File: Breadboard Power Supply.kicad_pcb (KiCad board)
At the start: 2 copper layers, 53.6 x 25.8 mm, 25 parts, among them J1 USB-C, J10 Conn_01x02_Male, J11 Conn_01x02_Male, J2 Conn_02x03_Odd_Even, J3 Conn_02x03_Odd_Even, J8 Conn_01x02_Male, J9 Conn_01x02_Male, U1 LM1117-1.8, U2 LM1117-3.3

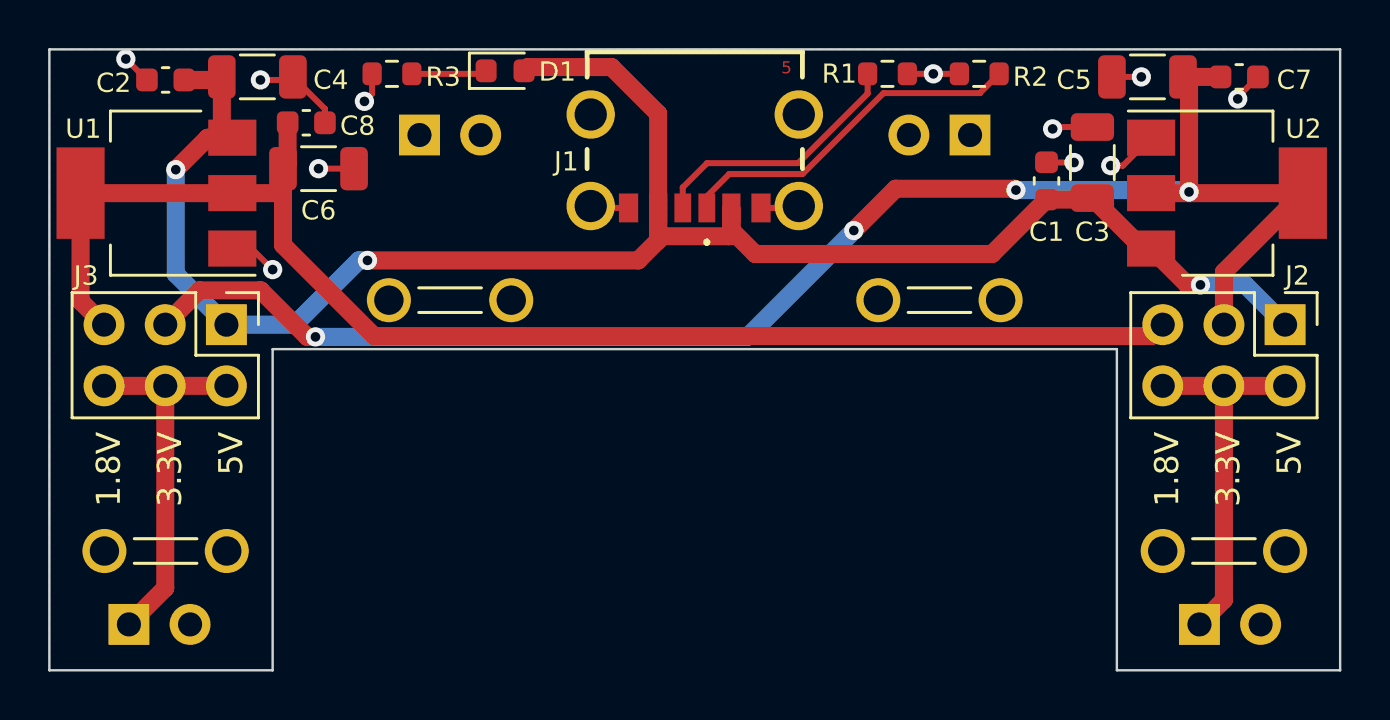
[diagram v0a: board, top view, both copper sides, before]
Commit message: Completed layout.
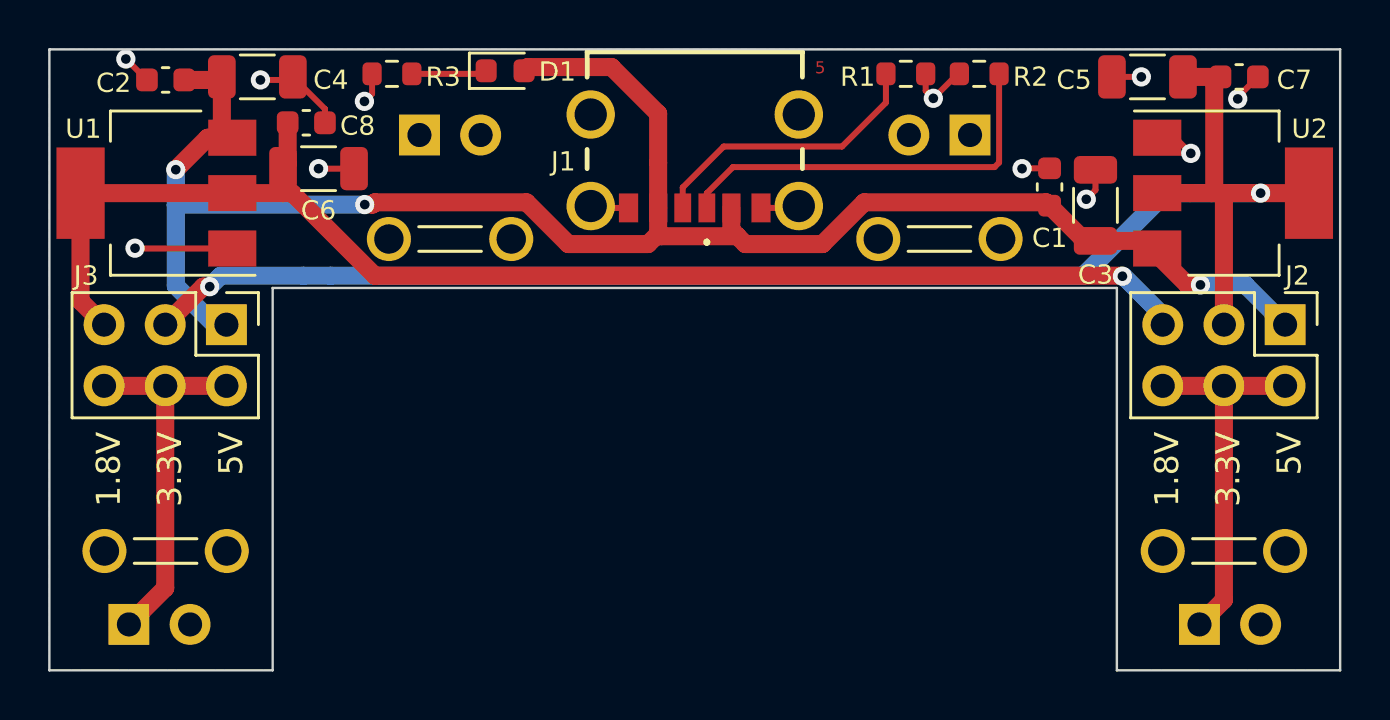
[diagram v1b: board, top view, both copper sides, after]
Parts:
- moved TP2 2.54 mm to (118.1, 83.1)
- moved TP3 2.54 mm to (138.4, 83.1)
- moved C3 1.78 mm to (144.9, 81.7)
- moved R1 0.76 mm to (137.0, 76.2)
- moved C1 0.28 mm to (143.0, 80.9)
- moved U2 0.25 mm to (150.6, 81.2)
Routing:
- net Net-(J1-CC1): track 14.7 -> 17.0 mm
- net GND: track 22.5 -> 24.7 mm
- net +1V8: track 57.7 -> 56.3 mm, vias 0 -> 1
- net +5V: track 78.6 -> 77.3 mm
- net Net-(J1-CC2): track 11.0 -> 11.9 mm
- net +3.3V: track 66.1 -> 66.0 mm, vias 4 -> 2
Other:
- outline, holes or cut-outs redrawn
